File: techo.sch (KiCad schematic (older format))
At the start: 24 parts, among them SW1 SW_Push, U1 ATmega32U4-AU, Y1 16MHz

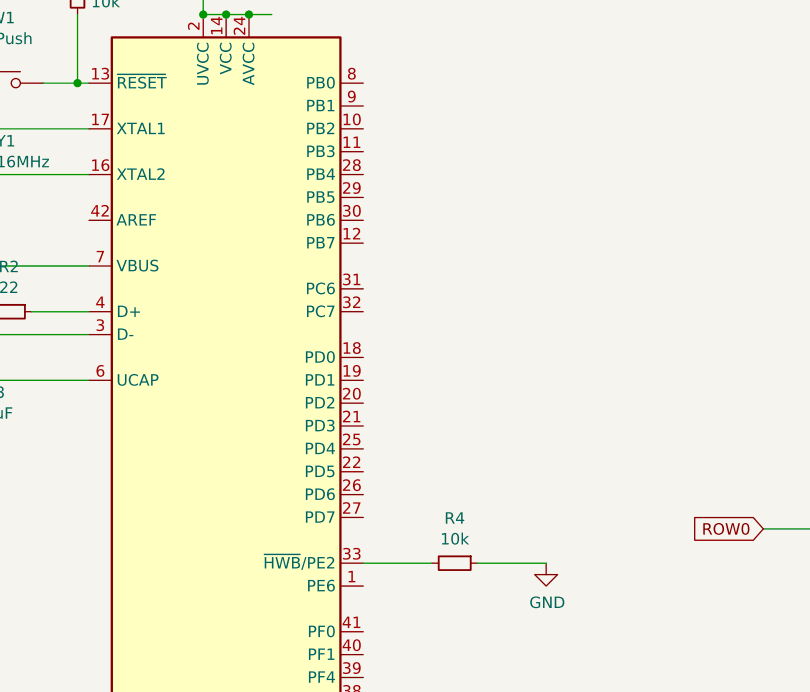
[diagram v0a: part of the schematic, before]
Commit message: Completed tutorial
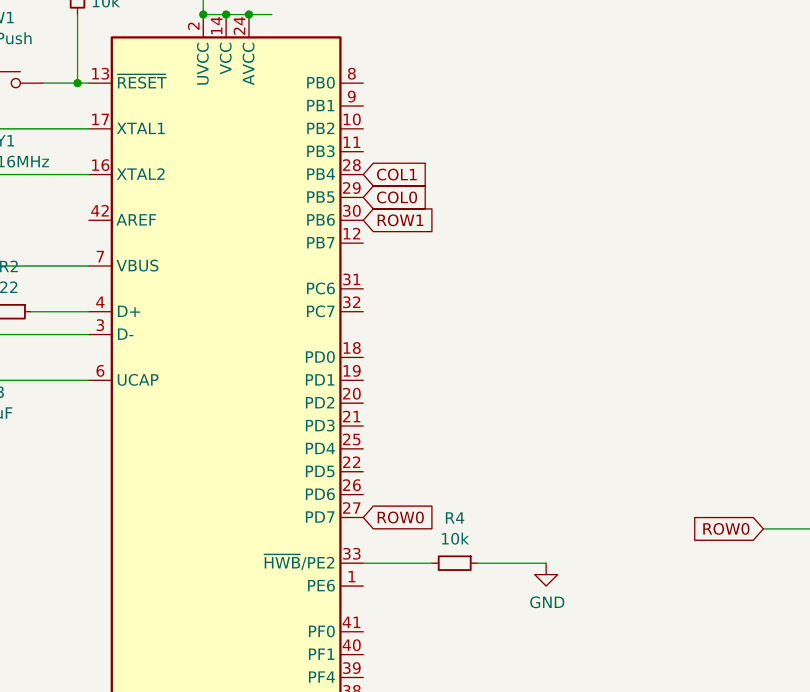
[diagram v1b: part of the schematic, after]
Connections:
- net COL0: now also U1.29 (PB5)
- net COL1: now also U1.28 (PB4)
- net ROW0: now also U1.27 (PD7)
- net ROW1: now also U1.30 (PB6)
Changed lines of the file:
@@
 Text GLabel 5200 4250 0    50   Input ~ 0
 ROW1
+Text GLabel 3500 1900 2    50   Input ~ 0
+COL1
+Text GLabel 3500 2000 2    50   Input ~ 0
+COL0
+Text GLabel 3500 2100 2    50   Input ~ 0
+ROW1
+Text GLabel 3500 3400 2    50   Input ~ 0
+ROW0
 $EndSCHEMATC
